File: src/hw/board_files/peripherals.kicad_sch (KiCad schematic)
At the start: 33 parts, among them J3 Screw_Terminal_01x03, J4 Molex 104031-0811, Q1 PMOS, U4 NEO-M9N, U5 BQ27411DRZT-G1A, U6 SHT30-DIS

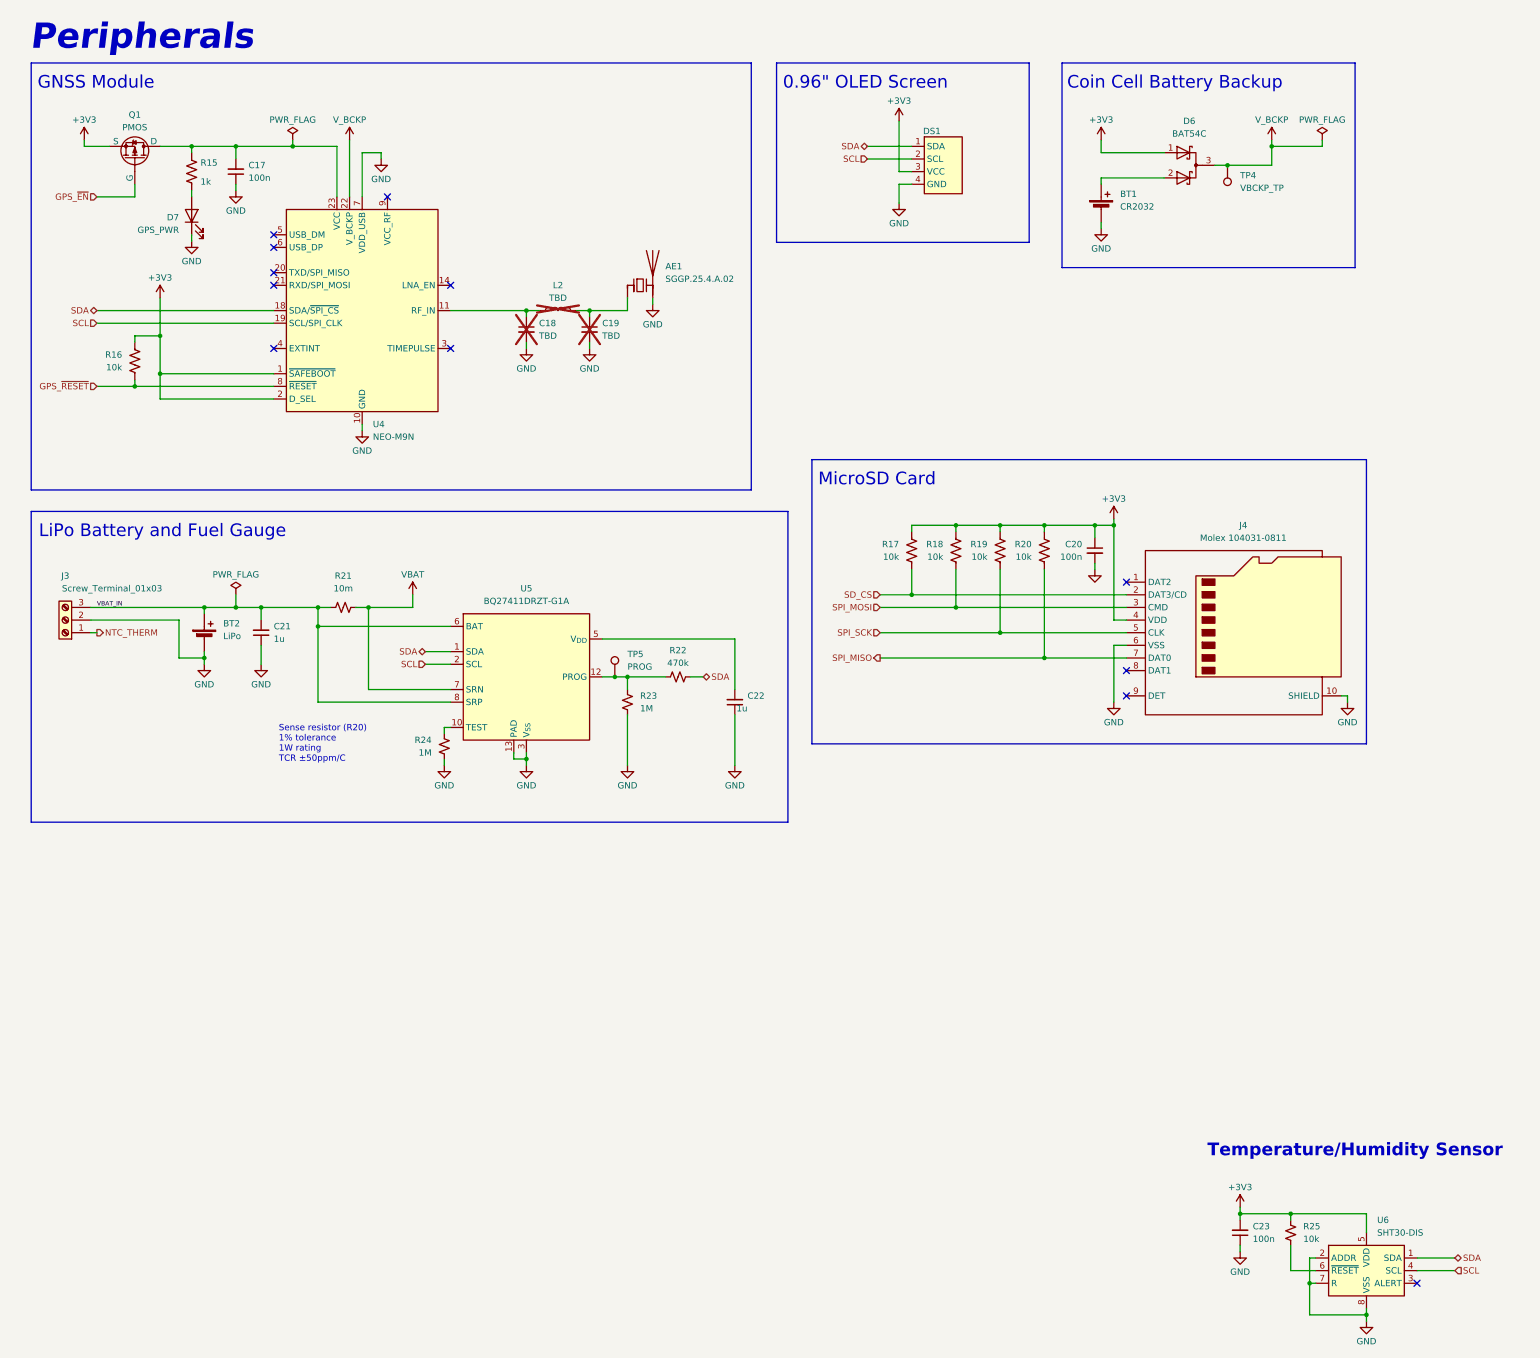
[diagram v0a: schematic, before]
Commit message: rev0.1 done
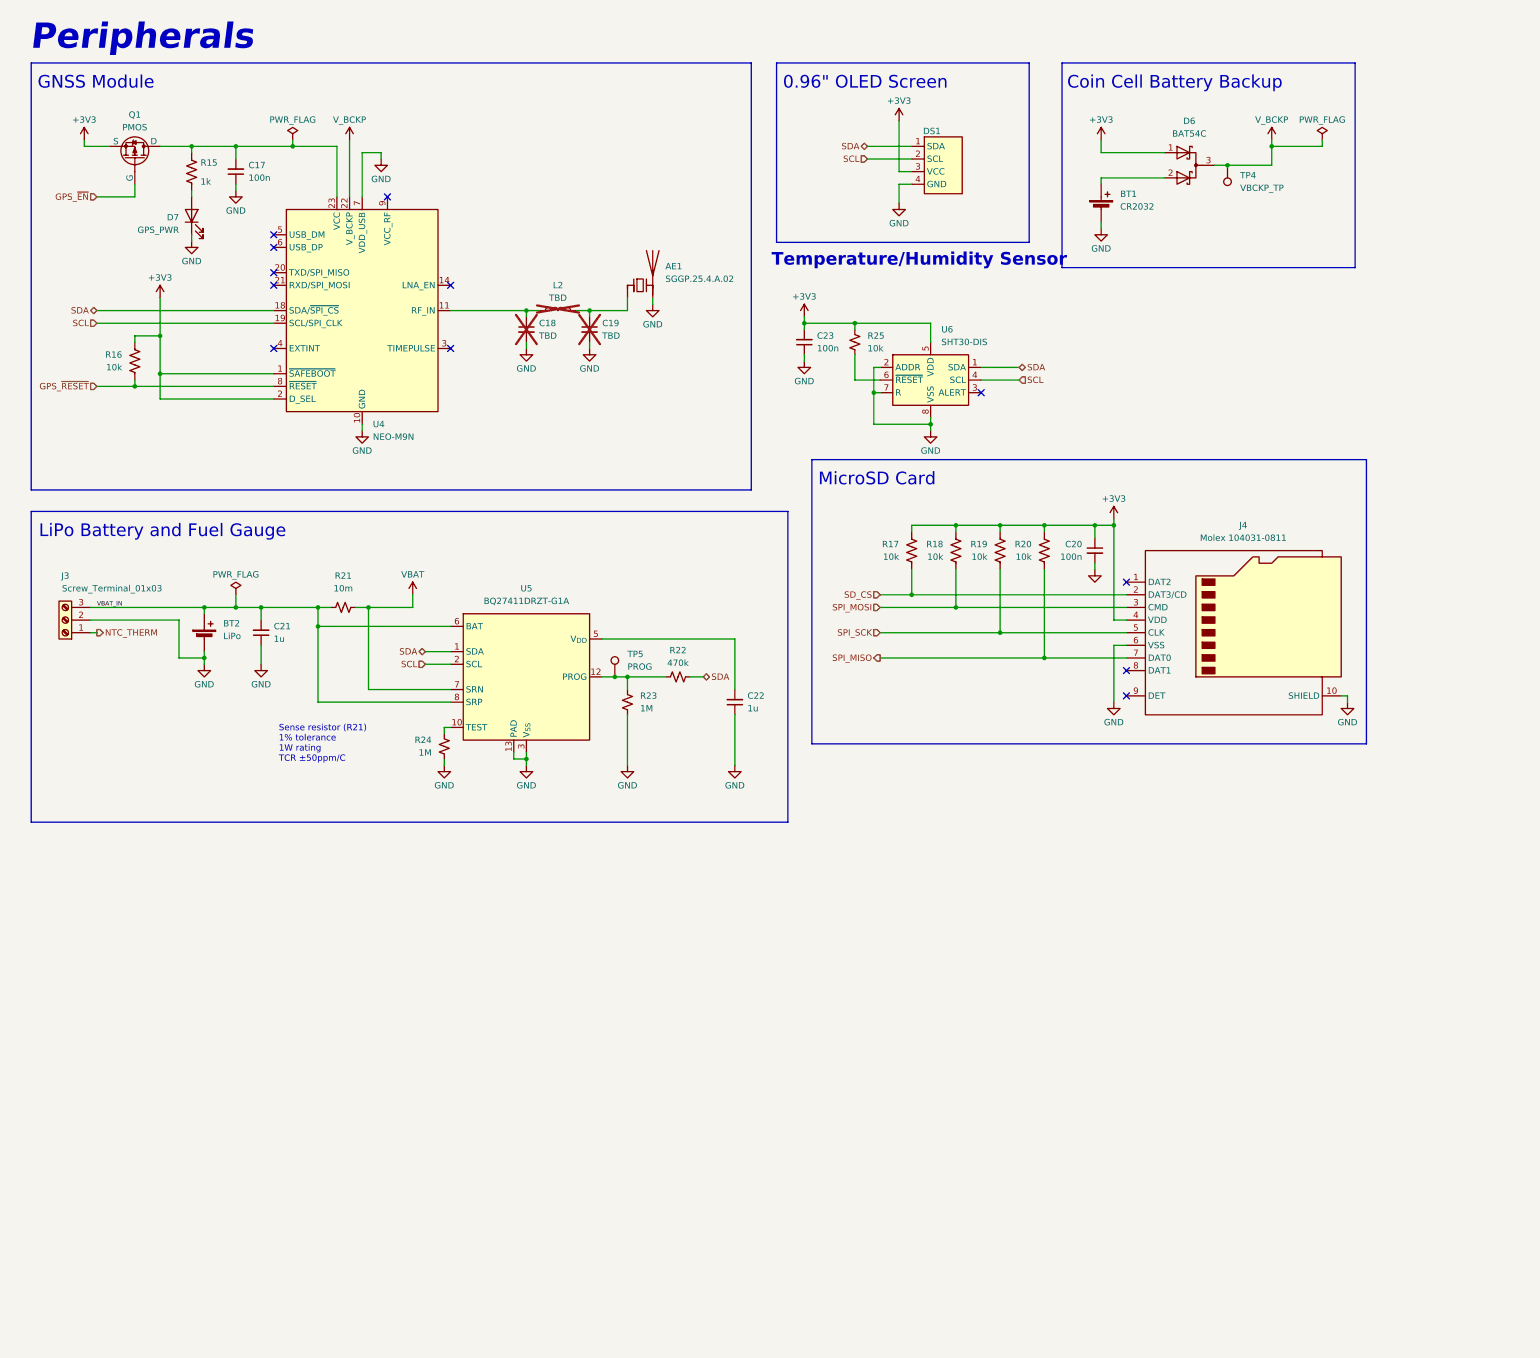
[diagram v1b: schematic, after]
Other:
- note added: "Sense resistor (R21) 1% tolerance 1W rating TCR ±50ppm/C"
- note removed: "Sense resistor (R20) 1% tolerance 1W rating TCR ±50ppm/C"
- moved on the sheet: C23, R25, U6
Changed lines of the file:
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@@
 		)
 	)
-	(text "Sense resistor (R20)\n1% tolerance\n1W rating\nTCR ±50ppm/C"
+	(text "Sense resistor (R21)\n1% tolerance\n1W rating\nTCR ±50ppm/C"
 		(exclude_from_sim no)
 		(at 64.516 160.782 0)
@@
 	(text "Temperature/Humidity Sensor"
 		(exclude_from_sim no)
-		(at 280.924 242.57 0)
+		(at 193.294 63.5 0)
 		(effects
 			(font
@@
 	)
 	(junction
-		(at 283.21 275.59)
+		(at 195.58 96.52)
 		(diameter 0)
 		(color 0 0 0 0)
@@
 	)
 	(junction
-		(at 271.78 269.24)
+		(at 184.15 90.17)
 		(diameter 0)
 		(color 0 0 0 0)
@@
 	)
 	(junction
-		(at 257.81 255.27)
+		(at 170.18 76.2)
 		(diameter 0)
 		(color 0 0 0 0)
@@
 	)
 	(junction
-		(at 267.97 255.27)
+		(at 180.34 76.2)
 		(diameter 0)
 		(color 0 0 0 0)
@@
 	)
 	(no_connect
-		(at 293.37 269.24)
+		(at 205.74 90.17)
 	)
 	(no_connect
@@
 	(wire
 		(pts
-			(xy 271.78 264.16) (xy 271.78 269.24)
+			(xy 184.15 85.09) (xy 184.15 90.17)
 		)
 		(stroke
@@
 	(wire
 		(pts
-			(xy 271.78 275.59) (xy 283.21 275.59)
+			(xy 184.15 96.52) (xy 195.58 96.52)
 		)
 		(stroke
@@
 	(wire
 		(pts
-			(xy 283.21 274.32) (xy 283.21 275.59)
+			(xy 195.58 95.25) (xy 195.58 96.52)
 		)
 		(stroke
@@
 	(wire
 		(pts
-			(xy 293.37 266.7) (xy 300.99 266.7)
+			(xy 205.74 87.63) (xy 213.36 87.63)
 		)
 		(stroke
@@
 	(wire
 		(pts
-			(xy 257.81 262.89) (xy 257.81 261.62)
+			(xy 170.18 83.82) (xy 170.18 82.55)
 		)
 		(stroke
@@
 	(wire
 		(pts
-			(xy 257.81 254) (xy 257.81 255.27)
+			(xy 170.18 74.93) (xy 170.18 76.2)
 		)
 		(stroke
@@
 	(wire
 		(pts
-			(xy 283.21 275.59) (xy 283.21 276.86)
+			(xy 195.58 96.52) (xy 195.58 97.79)
 		)
 		(stroke
@@
 	(wire
 		(pts
-			(xy 273.05 266.7) (xy 267.97 266.7)
+			(xy 185.42 87.63) (xy 180.34 87.63)
 		)
 		(stroke
@@
 	(wire
 		(pts
-			(xy 267.97 261.62) (xy 267.97 266.7)
+			(xy 180.34 82.55) (xy 180.34 87.63)
 		)
 		(stroke
@@
 	(wire
 		(pts
-			(xy 293.37 264.16) (xy 300.99 264.16)
+			(xy 205.74 85.09) (xy 213.36 85.09)
 		)
 		(stroke
@@
 	(wire
 		(pts
-			(xy 283.21 259.08) (xy 283.21 255.27)
+			(xy 195.58 80.01) (xy 195.58 76.2)
 		)
 		(stroke
@@
 	(wire
 		(pts
-			(xy 273.05 269.24) (xy 271.78 269.24)
+			(xy 185.42 90.17) (xy 184.15 90.17)
 		)
 		(stroke
@@
 	(wire
 		(pts
-			(xy 271.78 269.24) (xy 271.78 275.59)
+			(xy 184.15 90.17) (xy 184.15 96.52)
 		)
 		(stroke
@@
 	(wire
 		(pts
-			(xy 257.81 255.27) (xy 267.97 255.27)
+			(xy 170.18 76.2) (xy 180.34 76.2)
 		)
 		(stroke
@@
 	(wire
 		(pts
-			(xy 267.97 255.27) (xy 267.97 256.54)
+			(xy 180.34 76.2) (xy 180.34 77.47)
 		)
 		(stroke
@@
 	(wire
 		(pts
-			(xy 283.21 255.27) (xy 267.97 255.27)
+			(xy 195.58 76.2) (xy 180.34 76.2)
 		)
 		(stroke
@@
 	(wire
 		(pts
-			(xy 273.05 264.16) (xy 271.78 264.16)
+			(xy 185.42 85.09) (xy 184.15 85.09)
 		)
 		(stroke
@@
 	(wire
 		(pts
-			(xy 257.81 256.54) (xy 257.81 255.27)
+			(xy 170.18 77.47) (xy 170.18 76.2)
 		)
 		(stroke
@@
 	(hierarchical_label "SCL"
 		(shape input)
-		(at 300.99 266.7 0)
+		(at 213.36 87.63 0)
 		(effects
 			(font
@@
 	(hierarchical_label "SDA"
 		(shape bidirectional)
-		(at 300.99 264.16 0)
+		(at 213.36 85.09 0)
 		(effects
 			(font
@@
 	(symbol
 		(lib_id "Device:R_Small_US")
-		(at 267.97 259.08 0)
+		(at 180.34 80.01 0)
 		(unit 1)
 		(exclude_from_sim no)
@@
 		(fields_autoplaced yes)
 		(property "Reference" "R25"
-			(at 270.51 257.8099 0)
+			(at 182.88 78.7399 0)
 			(effects
 				(font
@@
 		)
 		(property "Value" "10k"
-			(at 270.51 260.3499 0)
+			(at 182.88 81.2799 0)
 			(effects
 				(font
@@
 		)
 		(property "Footprint" "Resistor_SMD:R_0603_1608Metric_Pad0.98x0.95mm_HandSolder"
-			(at 267.97 259.08 0)
+			(at 180.34 80.01 0)
 			(effects
 				(font
@@
 		)
 		(property "Datasheet" "~"
-			(at 267.97 259.08 0)
+			(at 180.34 80.01 0)
 			(effects
 				(font
@@
 		)
 		(property "Description" "Resistor, small US symbol"
-			(at 267.97 259.08 0)
+			(at 180.34 80.01 0)
 			(effects
 				(font
@@
 	(symbol
 		(lib_id "power:GND")
-		(at 257.81 262.89 0)
+		(at 170.18 83.82 0)
 		(unit 1)
 		(exclude_from_sim no)
@@
 		(dnp no)
 		(property "Reference" "#PWR074"
-			(at 257.81 269.24 0)
+			(at 170.18 90.17 0)
 			(effects
 				(font
@@
 		)
 		(property "Value" "GND"
-			(at 257.81 266.954 0)
+			(at 170.18 87.884 0)
 			(effects
 				(font
@@
 		)
 		(property "Footprint" ""
-			(at 257.81 262.89 0)
+			(at 170.18 83.82 0)
 			(effects
 				(font
@@
 		)
 		(property "Datasheet" ""
-			(at 257.81 262.89 0)
+			(at 170.18 83.82 0)
 			(effects
 				(font
@@
 		)
 		(property "Description" "Power symbol creates a global label with name \"GND\" , ground"
-			(at 257.81 262.89 0)
+			(at 170.18 83.82 0)
 			(effects
 				(font
@@
 	(symbol
 		(lib_id "power:GND")
-		(at 283.21 276.86 0)
+		(at 195.58 97.79 0)
 		(unit 1)
 		(exclude_from_sim no)
@@
 		(dnp no)
 		(property "Reference" "#PWR075"
-			(at 283.21 283.21 0)
+			(at 195.58 104.14 0)
 			(effects
 				(font
@@
 		)
 		(property "Value" "GND"
-			(at 283.21 280.924 0)
+			(at 195.58 101.854 0)
 			(effects
 				(font
@@
 		)
 		(property "Footprint" ""
-			(at 283.21 276.86 0)
+			(at 195.58 97.79 0)
 			(effects
 				(font
@@
 		)
 		(property "Datasheet" ""
-			(at 283.21 276.86 0)
+			(at 195.58 97.79 0)
 			(effects
 				(font
@@
 		)
 		(property "Description" "Power symbol creates a global label with name \"GND\" , ground"
-			(at 283.21 276.86 0)
+			(at 195.58 97.79 0)
 			(effects
 				(font
@@
 		(on_board yes)
 		(dnp no)
+		(fields_autoplaced yes)
 		(property "Reference" "C22"
 			(at 158.75 151.1235 0)
@@
 					(size 1.27 1.27)
 				)
-				(justify left)
+				(justify right)
 			)
 		)
@@
 	(symbol
 		(lib_id "Sensor_Humidity:SHT30-DIS")
-		(at 283.21 266.7 0)
+		(at 195.58 87.63 0)
 		(unit 1)
 		(exclude_from_sim no)
@@
 		(fields_autoplaced yes)
 		(property "Reference" "U6"
-			(at 285.3533 256.54 0)
+			(at 197.7233 77.47 0)
 			(effects
 				(font
@@
 		)
 		(property "Value" "SHT30-DIS"
-			(at 285.3533 259.08 0)
+			(at 197.7233 80.01 0)
 			(effects
 				(font
@@
 		)
 		(property "Footprint" "Sensor_Humidity:Sensirion_DFN-8-1EP_2.5x2.5mm_P0.5mm_EP1.1x1.7mm"
-			(at 283.21 265.43 0)
+			(at 195.58 86.36 0)
 			(effects
 				(font
@@
 		)
 		(property "Datasheet" "https://sensirion.com/media/documents/213E6A3B/63A5A569/Datasheet_SHT3x_DIS.pdf"
-			(at 283.21 265.43 0)
+			(at 195.58 86.36 0)
 			(effects
 				(font
@@
 		)
 		(property "Description" "I²C humidity and temperature sensor, ±2%RH, ±0.2°C, DFN-8"
-			(at 283.21 266.7 0)
+			(at 195.58 87.63 0)
 			(effects
 				(font
@@
 	(symbol
 		(lib_id "Device:C_Small")
-		(at 257.81 259.08 180)
+		(at 170.18 80.01 180)
 		(unit 1)
 		(exclude_from_sim no)
@@
 		(fields_autoplaced yes)
 		(property "Reference" "C23"
-			(at 260.35 257.8035 0)
+			(at 172.72 78.7335 0)
 			(effects
 				(font
@@
 		)
 		(property "Value" "100n"
-			(at 260.35 260.3435 0)
+			(at 172.72 81.2735 0)
 			(effects
 				(font
@@
 		)
 		(property "Footprint" "Capacitor_SMD:C_0603_1608Metric_Pad1.08x0.95mm_HandSolder"
-			(at 257.81 259.08 0)
+			(at 170.18 80.01 0)
 			(effects
 				(font
@@
 		)
 		(property "Datasheet" "~"
-			(at 257.81 259.08 0)
+			(at 170.18 80.01 0)
 			(effects
 				(font
@@
 		)
 		(property "Description" "Unpolarized capacitor, small symbol"
-			(at 257.81 259.08 0)
+			(at 170.18 80.01 0)
 			(effects
 				(font
@@
 	(symbol
 		(lib_id "power:+3V3")
-		(at 257.81 254 0)
+		(at 170.18 74.93 0)
 		(unit 1)
 		(exclude_from_sim no)
@@
 		(dnp no)
 		(property "Reference" "#PWR073"
-			(at 257.81 257.81 0)
+			(at 170.18 78.74 0)
 			(effects
 				(font
@@
 		)
 		(property "Value" "+3V3"
-			(at 257.81 249.936 0)
+			(at 170.18 70.866 0)
 			(effects
 				(font
@@
 		)
 		(property "Footprint" ""
-			(at 257.81 254 0)
+			(at 170.18 74.93 0)
 			(effects
 				(font
@@
 		)
 		(property "Datasheet" ""
-			(at 257.81 254 0)
+			(at 170.18 74.93 0)
 			(effects
 				(font
@@
 		)
 		(property "Description" "Power symbol creates a global label with name \"+3V3\""
-			(at 257.81 254 0)
+			(at 170.18 74.93 0)
 			(effects
 				(font
